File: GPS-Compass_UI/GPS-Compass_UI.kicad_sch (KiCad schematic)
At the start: 26 parts, among them J4 Conn_01x10_Socket, SW1 SPDT, SW3 RESET, SW4 EXT, SW5 RESET, SW6 EXT, SW7 EXT, SW8 EXT

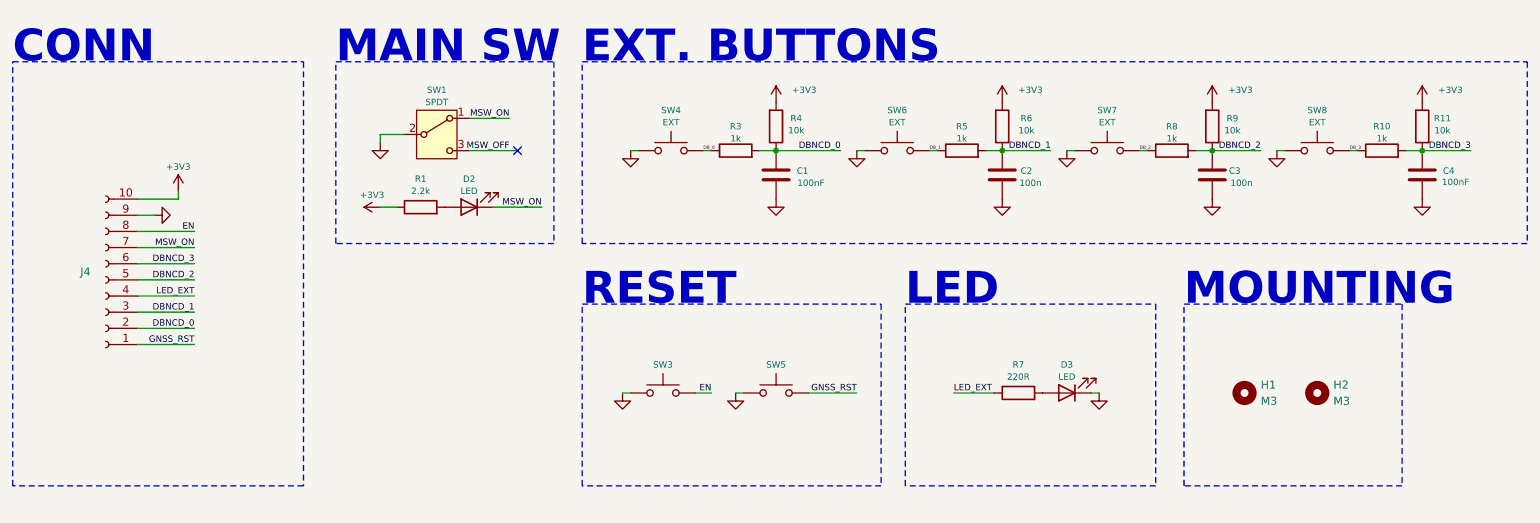
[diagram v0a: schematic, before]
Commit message: UI board updates
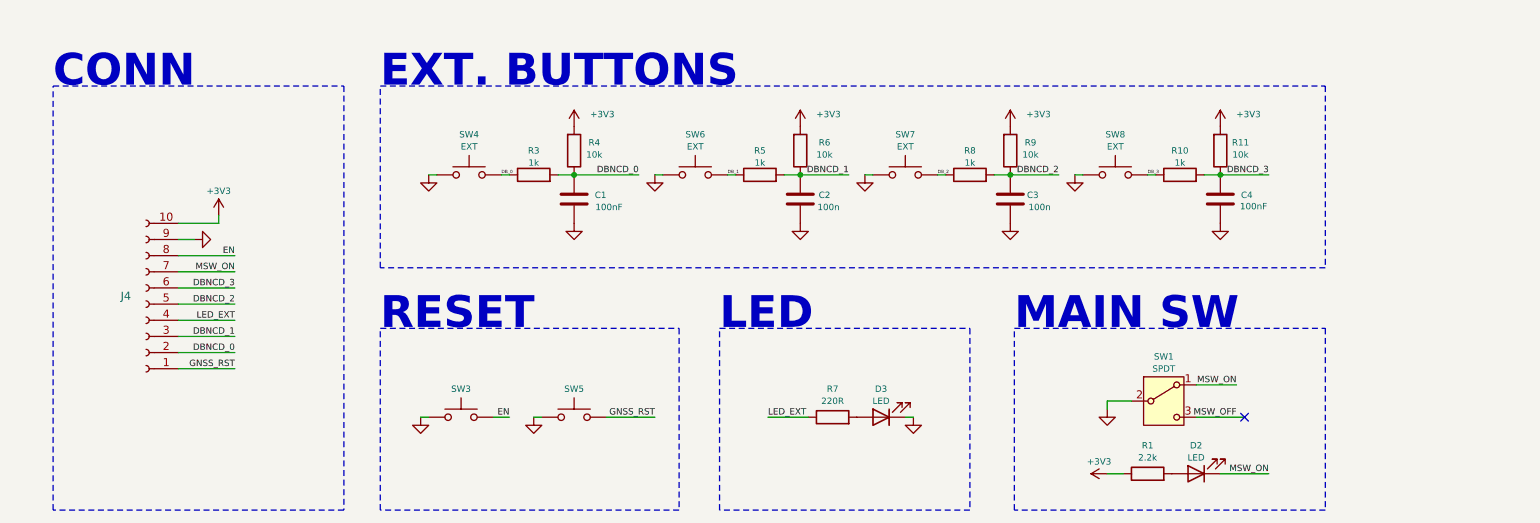
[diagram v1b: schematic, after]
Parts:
- removed H1, H2: M3, MountingHole:MountingHole_3.2mm_M3, symbol Mechanical:MountingHole
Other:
- note removed: "MOUNTING"
- moved on the sheet: C1, C2, C3, C4, D2, D3, J4, R1, R10, R11, R3, R4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
